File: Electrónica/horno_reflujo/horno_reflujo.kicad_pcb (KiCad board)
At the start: 2 copper layers, 39 parts, among them J2 5V USB cargador, J3 Nextion_touch_screen, J4 Max6675_modulo, J5 ESP01, J6 Alimentación y zc, J7 Relevador a ventilador, J8 Tarjeta a SSR, J9 SSR a resistencias, K1 SANYOU_SRD_Form_C, Q1 2N2222A-TO92, U1 SSR-40 DA, U2 LM7805CT, U3 74LS14, U4 LM7833CT, U5 ESP-01S

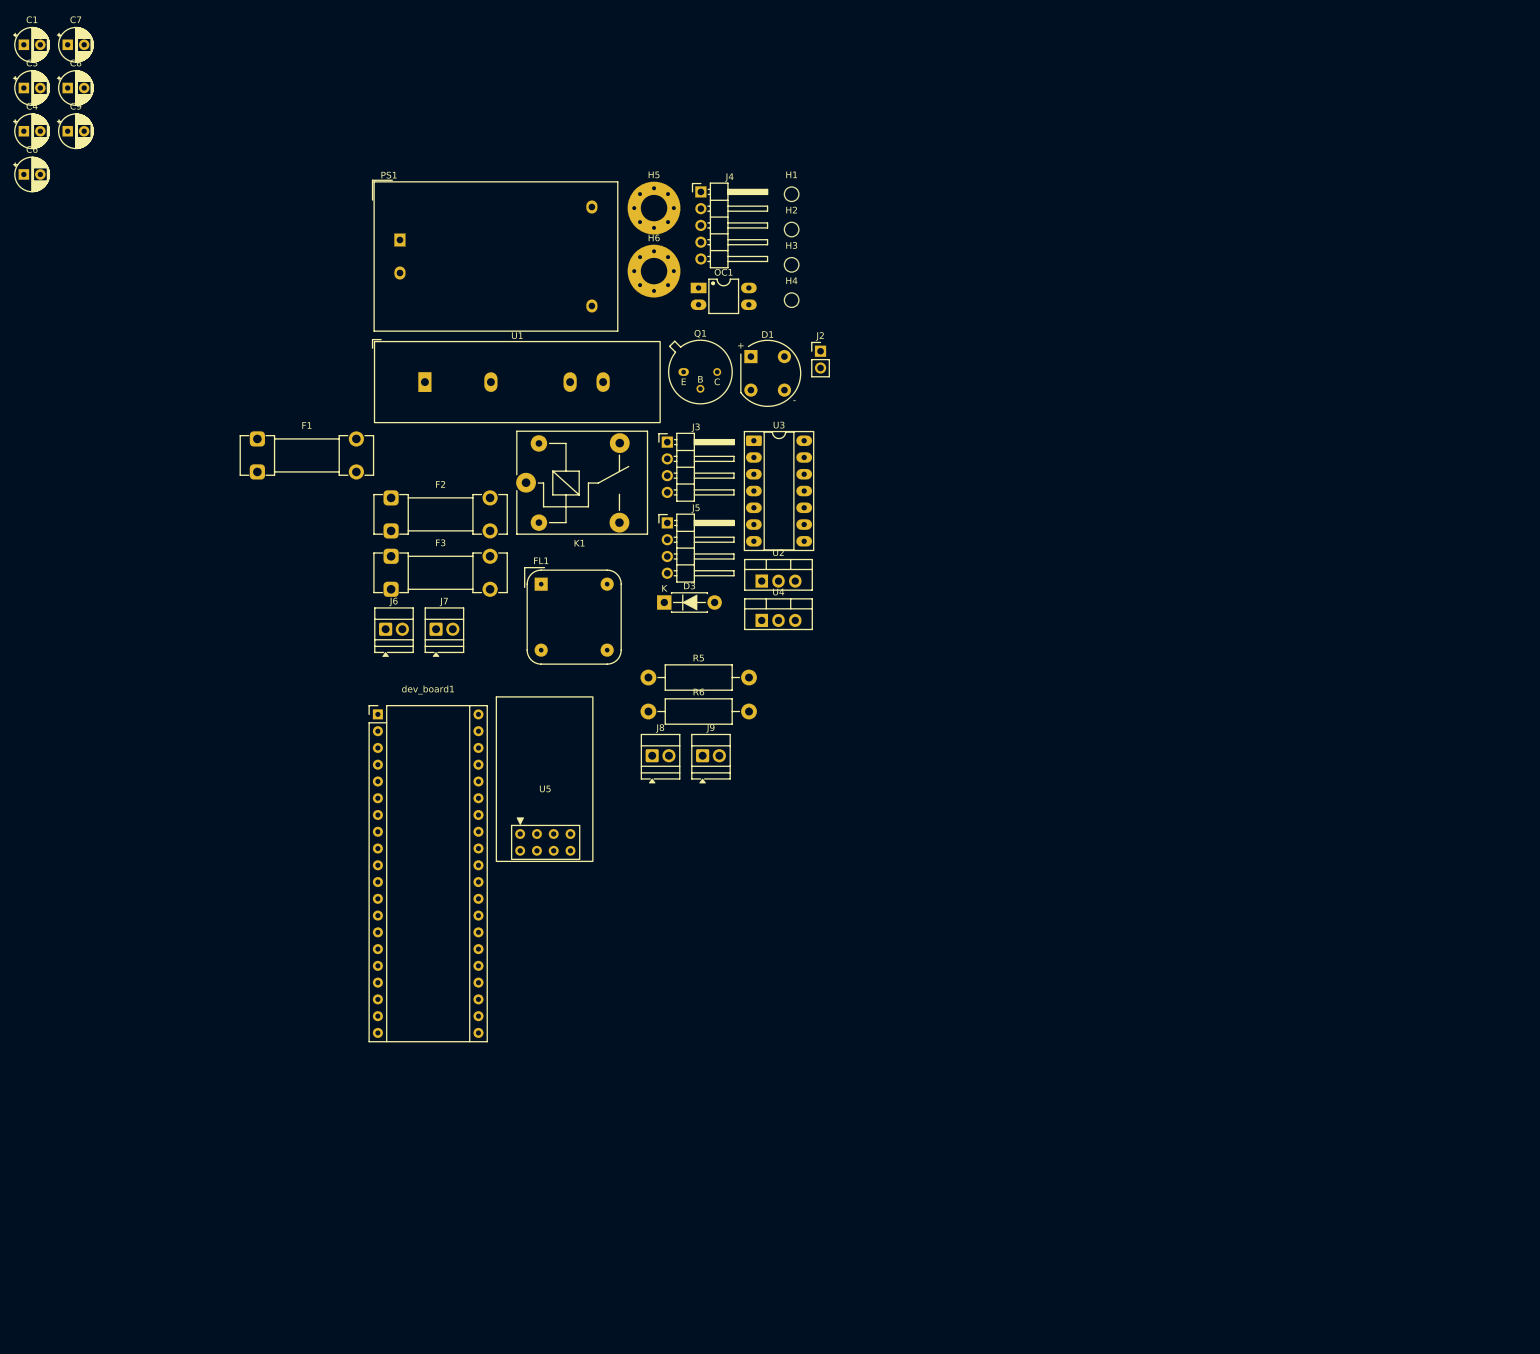
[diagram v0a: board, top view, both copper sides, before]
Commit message: pcb updated :)
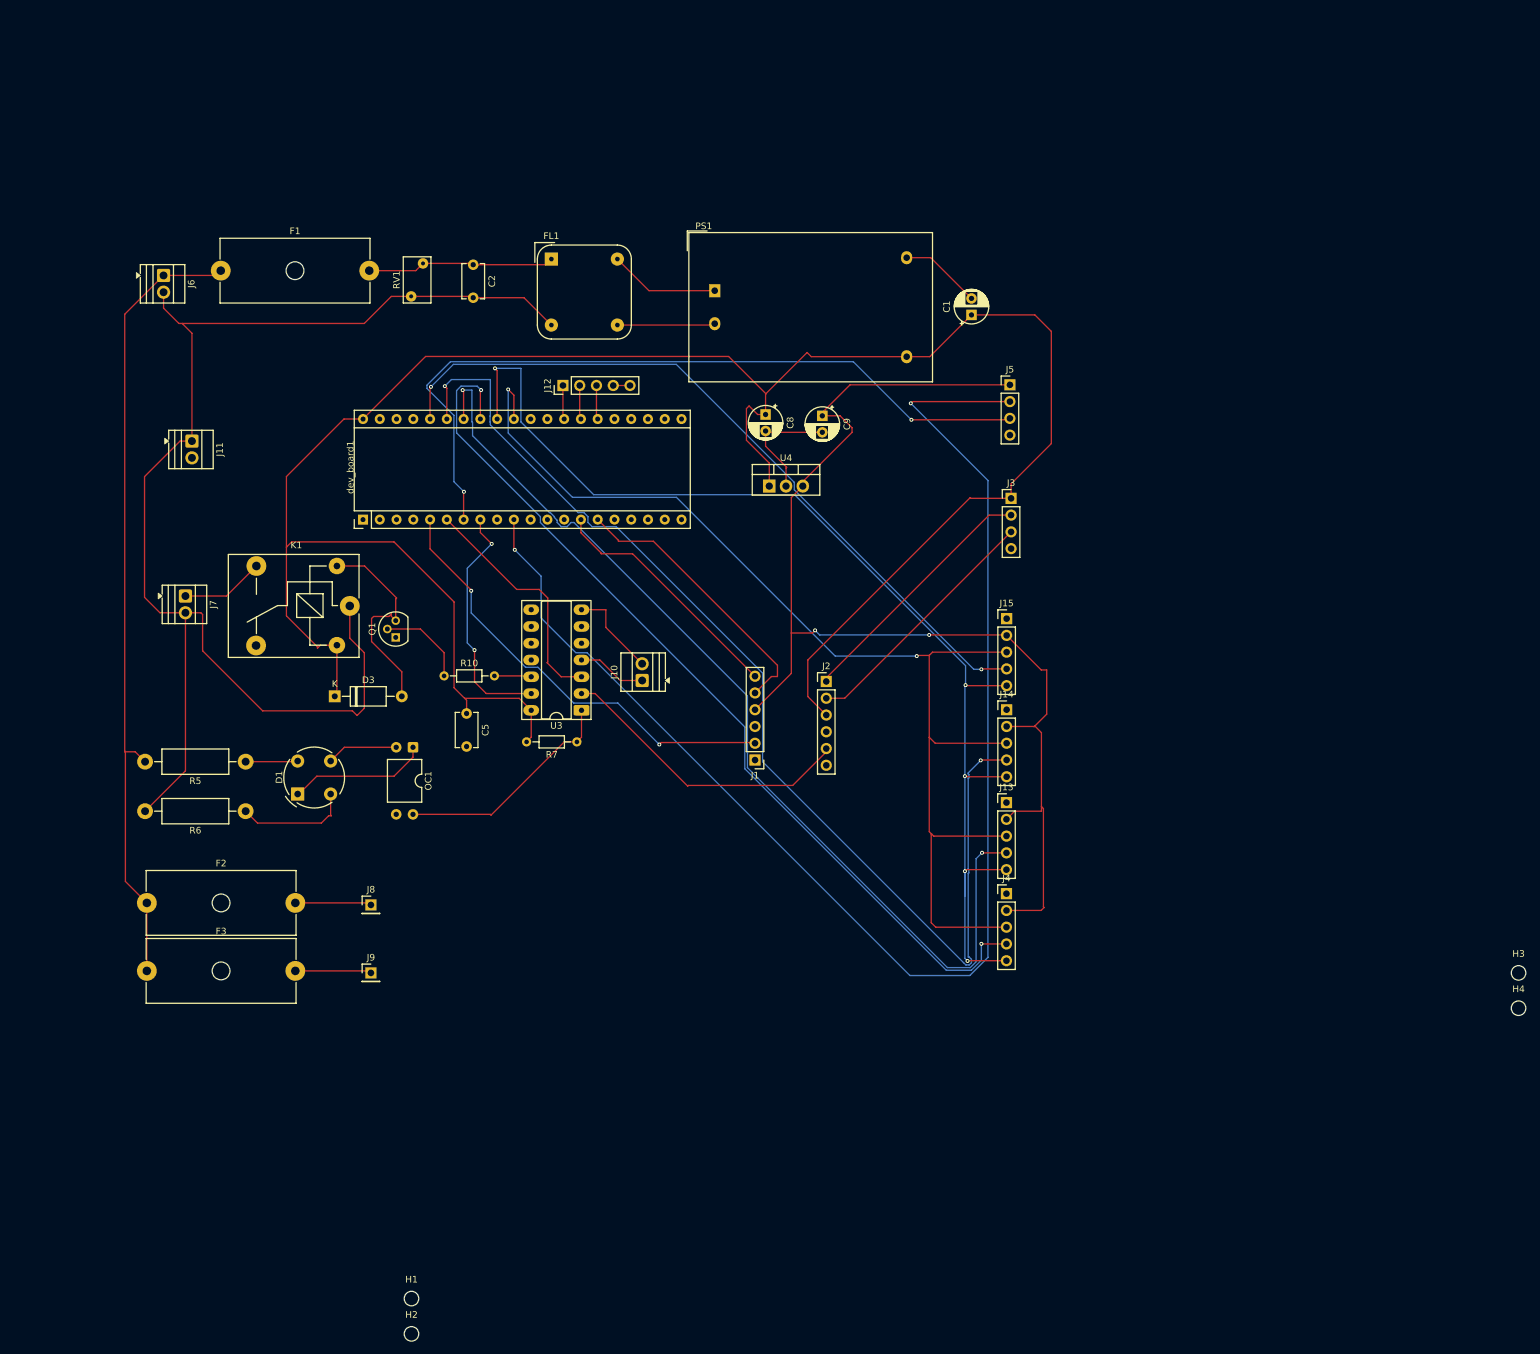
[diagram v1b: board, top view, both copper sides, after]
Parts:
- removed C3, C7: 1uf, Capacitor_THT:CP_Radial_D5.0mm_P2.50mm
- removed C4, C6: 10uf, Capacitor_THT:CP_Radial_D5.0mm_P2.50mm
- removed H5, H6: MountingHole_Pad_MP, MountingHole:MountingHole_4mm_Pad_Via
- removed U1: SSR-40 DA, Relay_THT:Relay_NCR_HHG1D-1
- removed U2: LM7805CT, PCM_Package_TO_SOT_THT_AKL:TO-220-3_Vertical
- removed U5: ESP-01S, RF_Module:ESP-01
- added C2: 0.1uF/275Vac, Capacitor_THT:C_Disc_D5.1mm_W3.2mm_P5.00mm, F.Cu at (69.7, 36.1)
- added C5: 100nf, Capacitor_THT:C_Disc_D5.1mm_W3.2mm_P5.00mm, F.Cu at (68.7, 104.1)
- added J1: LevelShifter, Connector_PinHeader_2.54mm:PinHeader_1x06_P2.54mm_Vertical, F.Cu at (112.4, 111.2)
- added J10: ssr1, TerminalBlock:TerminalBlock_Xinya_XY308-2.54-2P_1x02_P2.54mm_Horizontal, F.Cu at (95.3, 99.1)
- added J11: ssr2, TerminalBlock:TerminalBlock_Xinya_XY308-2.54-2P_1x02_P2.54mm_Horizontal, F.Cu at (27.1, 62.8)
- added J12: encoder, Connector_PinHeader_2.54mm:PinHeader_1x05_P2.54mm_Vertical, F.Cu at (83.3, 54.4)
- added J13: Max6675_modulo2, Connector_PinHeader_2.54mm:PinHeader_1x05_P2.54mm_Vertical, F.Cu at (150.5, 117.6)
- added J14: Max6675_modulo3, Connector_PinHeader_2.54mm:PinHeader_1x05_P2.54mm_Vertical, F.Cu at (150.5, 103.5)
- added J15: Max6675_modulo4, Connector_PinHeader_2.54mm:PinHeader_1x05_P2.54mm_Vertical, F.Cu at (150.5, 89.7)
- added R10: 1K, Resistor_THT:R_Axial_DIN0204_L3.6mm_D1.6mm_P7.62mm_Horizontal, F.Cu at (65.3, 98.4)
- added R7: 10K, Resistor_THT:R_Axial_DIN0204_L3.6mm_D1.6mm_P7.62mm_Horizontal, F.Cu at (85.4, 108.4)
- added RV1: 10D561K, Varistor:RV_Disc_D7mm_W4.2mm_P5mm, F.Cu at (62.1, 35.9)
- D1: footprint PCM_Diode_THT_AKL:Diode_Bridge_Round_D9.8mm -> Diode_THT:Diode_Bridge_Round_D9.0mm
- D3: footprint PCM_Diode_THT_AKL:D_DO-41_SOD81_P7.62mm_Horizontal -> Diode_THT:D_A-405_P10.16mm_Horizontal
- F1, F2, F3: footprint Fuse:Fuseholder_Clip-5x20mm_Schurter_OG_Lateral_P15.00x5.00mm_D1.3mm_Horizontal -> Fuse:Fuseholder_Cylinder-5x20mm_Schurter_0031_8201_Horizontal_Open
- J2: value 5V USB cargador -> LevelShifter; footprint Connector_PinHeader_2.54mm:PinHeader_1x02_P2.54mm_Vertical -> Connector_PinHeader_2.54mm:PinHeader_1x06_P2.54mm_Vertical
- J3: value Nextion_touch_screen -> Display Oled I2C; footprint Connector_PinHeader_2.54mm:PinHeader_1x04_P2.54mm_Horizontal -> Connector_PinHeader_2.54mm:PinHeader_1x04_P2.54mm_Vertical
- J4: footprint Connector_PinHeader_2.54mm:PinHeader_1x05_P2.54mm_Horizontal -> Connector_PinHeader_2.54mm:PinHeader_1x05_P2.54mm_Vertical
- J5: footprint Connector_PinHeader_2.54mm:PinHeader_1x04_P2.54mm_Horizontal -> Connector_PinHeader_2.54mm:PinHeader_1x04_P2.54mm_Vertical
- J8: value Tarjeta a SSR -> resistencia; footprint TerminalBlock:TerminalBlock_Xinya_XY308-2.54-2P_1x02_P2.54mm_Horizontal -> Connector_PinHeader_2.54mm:PinHeader_1x01_P2.54mm_Vertical
- J9: value SSR a resistencias -> resistencia1; footprint TerminalBlock:TerminalBlock_Xinya_XY308-2.54-2P_1x02_P2.54mm_Horizontal -> Connector_PinHeader_2.54mm:PinHeader_1x01_P2.54mm_Vertical
- OC1: footprint PCM_Package_DIP_AKL:DIP-4_W7.62mm_LongPads -> Package_DIP:DIP-4_W10.16mm
- Q1: footprint PCM_Package_TO_SOT_THT_AKL:TO-39-3_EBC -> Package_TO_SOT_THT:TO-92
- U4: footprint PCM_Package_TO_SOT_THT_AKL:TO-220-3_Vertical -> Package_TO_SOT_THT:TO-220-3_Vertical
- moved H1 177.0 mm to (60.4, 192.8)
- moved H2 177.0 mm to (60.4, 198.1)
- moved H3 153.8 mm to (228.1, 143.4)
- moved H4 153.8 mm to (228.1, 148.8)
- moved C1 149.3 mm to (145.2, 43.7), turned to 90 degrees
- moved C9 122.2 mm to (122.6, 59.0), turned to -90 degrees
- moved C8 116.7 mm to (114.0, 58.8), turned to -90 degrees
- moved J4 116.0 mm to (150.5, 131.4)
- moved D1 95.4 mm to (43.1, 116.3), turned to 90 degrees
- moved OC1 82.0 mm to (60.6, 109.2), turned to -90 degrees
- moved F3 72.9 mm to (20.2, 143.1)
- moved F2 71.7 mm to (20.2, 132.8)
- moved J6 63.3 mm to (22.8, 37.7), turned to -90 degrees
- moved R6 62.9 mm to (35.2, 118.9), turned to 180 degrees
- moved R5 62.3 mm to (35.2, 111.4), turned to 180 degrees
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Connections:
- F2 pad 2: Net-(F2-Pad2) -> Net-(J8-Pin_1)
- F3 pad 2: Net-(F3-Pad2) -> Net-(J9-Pin_1)
- J2 pad 1: GND -> Net-(J2-Pin_1)
- J2 pad 2: +5V -> Net-(J2-Pin_2)
- J3 pad 2: Net-(J3-Pin_2) -> Net-(J2-Pin_1)
- J3 pad 3: Net-(J3-Pin_3) -> Net-(J2-Pin_2)
- J4 pad 2: +5V -> +3.3V
- J4 pad 3: /sck -> SPI1_SCK
- J4 pad 4: /cs -> CS_0
- J4 pad 5: /so -> SPI1_MISO
- J8 pad 1: /SSR_led -> Net-(J8-Pin_1)
- J9 pad 1: unconnected-(J9-Pin_1-Pad1) -> Net-(J9-Pin_1)
- U3 pad 10: unconnected-(U3-Pad10) -> (no net)
- U3 pad 11: GND -> (no net)
- U3 pad 2: Net-(R8-Pad2) -> zero
- U3 pad 4: /SSR_led -> Net-(J10-Pin_1)
- U3 pad 5: /Tx_mcu_screen -> (no net)
- U3 pad 6: Net-(U3-Pad6) -> (no net)
- U3 pad 8: Net-(J3-Pin_3) -> (no net)
- U3 pad 9: Net-(U3-Pad6) -> (no net)
- dev_board1 pad 10: unconnected-(dev_board1-A15-Pad10) -> /Rx_mcu_esp01
- dev_board1 pad 14: unconnected-(dev_board1-B6-Pad14) -> I2C1_SCL
- dev_board1 pad 15: unconnected-(dev_board1-B7-Pad15) -> I2C1_SDA
- dev_board1 pad 22: unconnected-(dev_board1-C13-Pad22) -> built_in_led
- dev_board1 pad 26: unconnected-(dev_board1-A0-Pad26) -> ENCODER_A
- dev_board1 pad 27: unconnected-(dev_board1-A1-Pad27) -> ENCODER_B
- dev_board1 pad 28: unconnected-(dev_board1-A2-Pad28) -> ENCODER_BTN
- dev_board1 pad 31: unconnected-(dev_board1-A5-Pad31) -> SPI1_SCK
- dev_board1 pad 32: unconnected-(dev_board1-A6-Pad32) -> SPI1_MISO
- dev_board1 pad 33: unconnected-(dev_board1-A7-Pad33) -> CS_0
- dev_board1 pad 34: unconnected-(dev_board1-B0-Pad34) -> CS_1
- dev_board1 pad 35: unconnected-(dev_board1-B1-Pad35) -> CS_2
- dev_board1 pad 36: unconnected-(dev_board1-B2-Pad36) -> CS_3
- dev_board1 pad 5: unconnected-(dev_board1-A8-Pad5) -> /zc
- dev_board1 pad 6: unconnected-(dev_board1-A9-Pad6) -> /fire
- dev_board1 pad 7: unconnected-(dev_board1-A10-Pad7) -> /Tx_mcu_esp01
- dev_board1 pad 8: unconnected-(dev_board1-A11-Pad8) -> /fan
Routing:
- net +5V: track 0.00 -> 332.7 mm
- net /Rx_mcu_esp01: track 0.00 -> 211.8 mm, vias 0 -> 2
- net NEUT: track 0.00 -> 205.2 mm
- net +3.3V: track 0.00 -> 180.1 mm, vias 0 -> 2
- net SPI1_SCK: track 0.00 -> 177.1 mm, vias 0 -> 2
- net SPI1_MISO: track 0.00 -> 176.2 mm, vias 0 -> 5
- net CS_2: track 0.00 -> 170.5 mm, vias 0 -> 2
- net CS_1: track 0.00 -> 150.6 mm, vias 0 -> 2
- net CS_0: track 0.00 -> 139.5 mm, vias 0 -> 2
- net LINE: track 0.00 -> 122.0 mm
- net /Tx_mcu_esp01: track 0.00 -> 116.2 mm, vias 0 -> 2
- net CS_3: track 0.00 -> 113.4 mm, vias 0 -> 2
- net /zc: track 0.00 -> 68.6 mm, vias 0 -> 2
- net GND: track 0.00 -> 47.5 mm
- net zero: track 0.00 -> 45.3 mm
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
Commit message: actualización del main
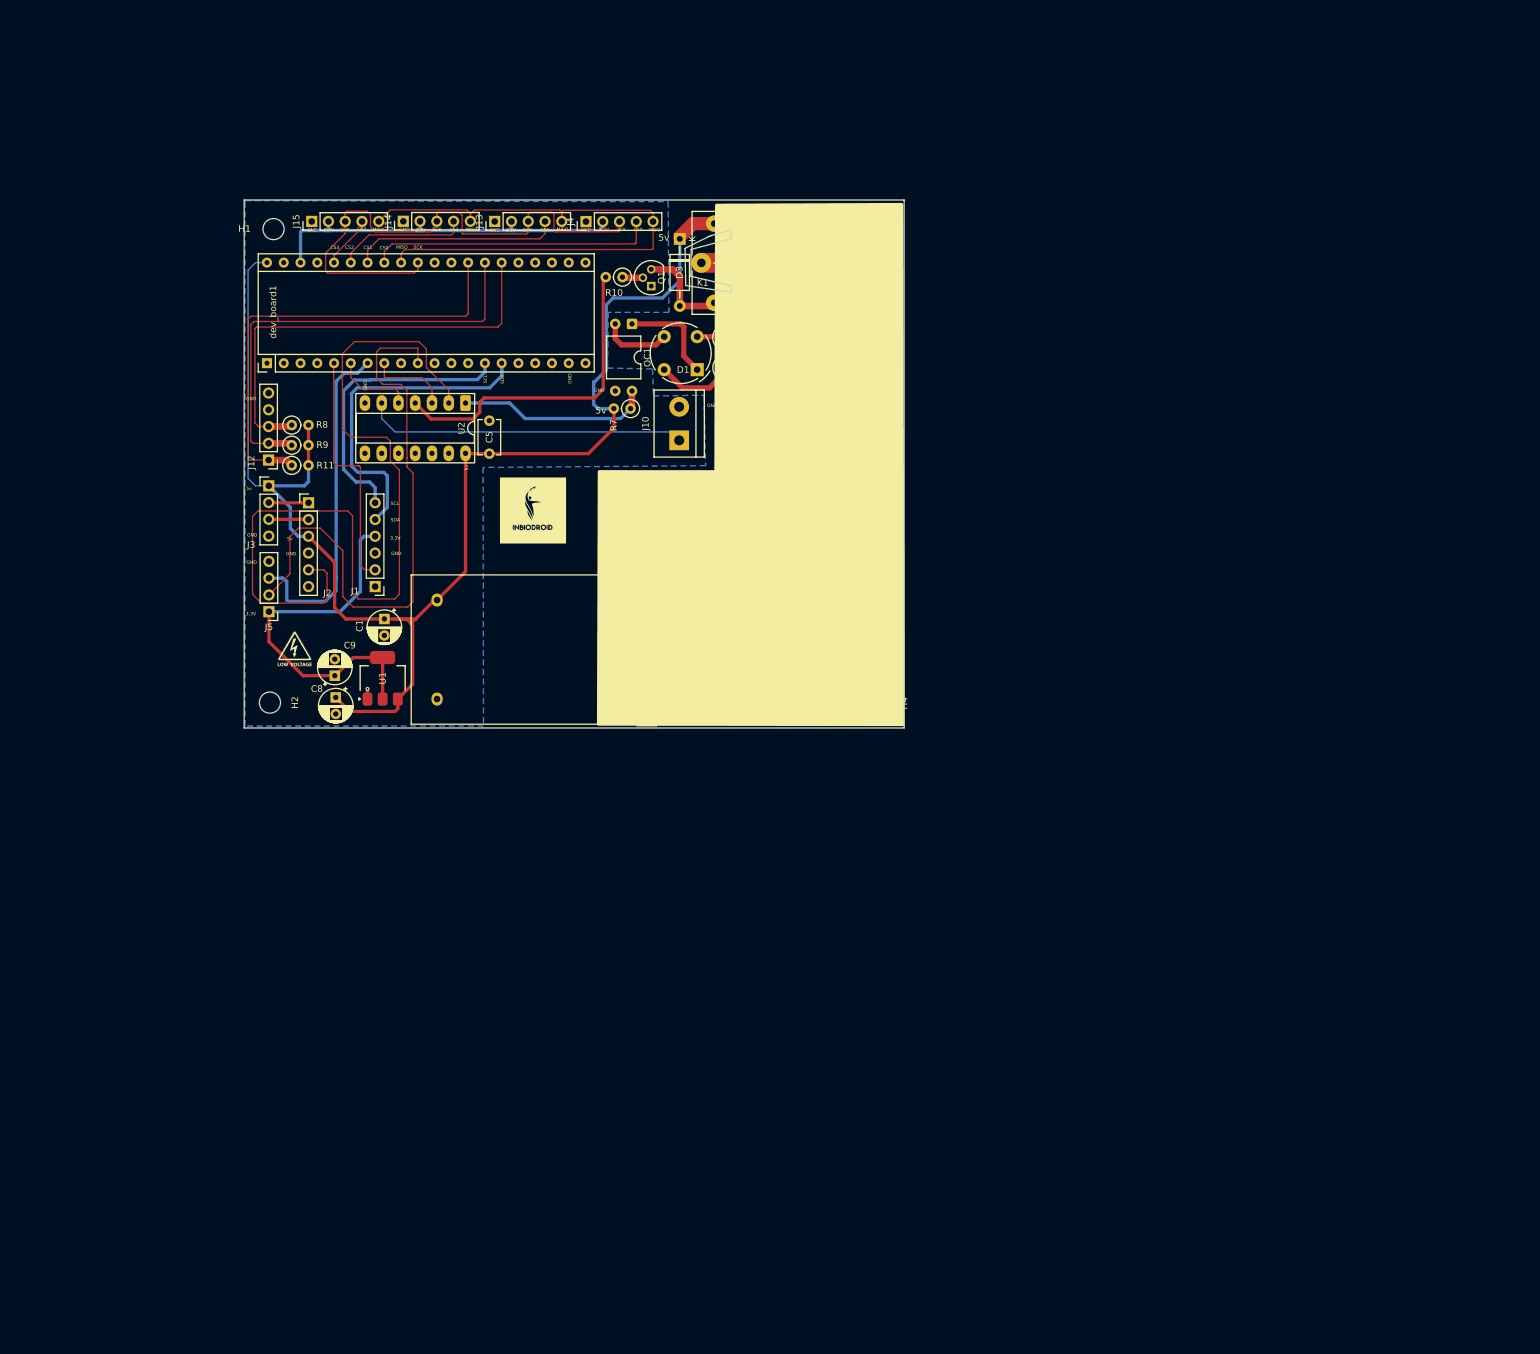
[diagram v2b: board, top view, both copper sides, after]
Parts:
- removed F3: 15A, Fuse:Fuseholder_Cylinder-5x20mm_Schurter_0031_8201_Horizontal_Open
- removed J9: resistencia1, Connector_PinHeader_2.54mm:PinHeader_1x01_P2.54mm_Vertical
- removed U3: 74LS14, Package_DIP:DIP-14_W7.62mm_Socket_LongPads
- removed U4: LM7833CT, Package_TO_SOT_THT:TO-220-3_Vertical
- added G***: LOGO, LOGO, F.Cu at (97.5, 74.9)
- added G***: LOGO, LOGO, F.Cu at (78.8, 73.3)
- added G***: LOGO, LOGO, F.Cu at (42.5, 94.2)
- added R11: 10K, Resistor_THT:R_Axial_DIN0207_L6.3mm_D2.5mm_P2.54mm_Vertical, F.Cu at (42.2, 66.5)
- added R8: 10K, Resistor_THT:R_Axial_DIN0207_L6.3mm_D2.5mm_P2.54mm_Vertical, F.Cu at (42.2, 60.4)
- added R9: 10K, Resistor_THT:R_Axial_DIN0207_L6.3mm_D2.5mm_P2.54mm_Vertical, F.Cu at (42.2, 63.5)
- added U1: LD1117S33TR_SOT223, Package_TO_SOT_SMD:SOT-223-3_TabPin2, F.Cu at (56.0, 98.8)
- added U2: 74LS14, Package_DIP:DIP-14_W7.62mm_Socket_LongPads, F.Cu at (68.5, 57.1)
- H1, H2, H3, H4: footprint MountingHole:MountingHole_2.2mm_M2_DIN965 -> MountingHole:MountingHole_3.2mm_M3_DIN965
- J10, J11, J6, J7: footprint TerminalBlock:TerminalBlock_Xinya_XY308-2.54-2P_1x02_P2.54mm_Horizontal -> TerminalBlock:TerminalBlock_bornier-2_P5.08mm
- R10, R7: footprint Resistor_THT:R_Axial_DIN0204_L3.6mm_D1.6mm_P7.62mm_Horizontal -> Resistor_THT:R_Axial_DIN0207_L6.3mm_D2.5mm_P2.54mm_Vertical
- R5, R6: footprint Resistor_THT:R_Axial_DIN0411_L9.9mm_D3.6mm_P15.24mm_Horizontal -> Resistor_THT:R_Axial_DIN0411_L9.9mm_D3.6mm_P5.08mm_Vertical
- moved H1 163.4 mm to (39.5, 30.7), turned to 180 degrees
- moved H3 148.6 mm to (131.8, 30.3), turned to 180 degrees
- moved F2 128.8 mm to (133.3, 71.2), turned to 180 degrees
- moved J6 122.6 mm to (130.9, 95.6), turned to 90 degrees
- moved J15 121.3 mm to (45.2, 29.5), turned to 90 degrees
- moved J4 120.1 mm to (86.8, 29.6), turned to 90 degrees
- moved J14 117.6 mm to (59.1, 29.5), turned to 90 degrees
- moved J5 117.4 mm to (38.8, 88.7), turned to 180 degrees
- moved J13 117.3 mm to (73.0, 29.5), turned to 90 degrees
- moved J7 112.5 mm to (127.0, 36.4)
- moved J3 112.5 mm to (38.7, 69.6)
- moved F1 111.2 mm to (133.3, 81.6), turned to 180 degrees
- moved H4 107.3 mm to (131.2, 102.5), turned to -90 degrees
- moved R6 102.1 mm to (107.9, 47.2), turned to 0 degrees
- moved C1 100.2 mm to (56.2, 89.8), turned to -90 degrees
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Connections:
- J13 pad 2: +3.3V -> +3.3Vmc
- J14 pad 2: +3.3V -> +3.3Vmc
- J15 pad 2: +3.3V -> +3.3Vmc
- J4 pad 2: +3.3V -> +3.3Vmc
- J6 pad 1: LINE -> NEUT
- J6 pad 2: NEUT -> LINE
- J7 pad 2: NEUT -> LINE
- R5 pad 2: LINE -> Net-(J8-Pin_1)
- dev_board1 pad 38: unconnected-(dev_board1-3.3-Pad38) -> +3.3Vmc
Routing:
- net CS_2: track 170.5 -> 20.0 mm, vias 2 -> 0
- net /Rx_mcu_esp01: track 211.8 -> 89.3 mm, vias 2 -> 0
- net +3.3V: track 180.1 -> 57.8 mm, vias 2 -> 0
- net CS_1: track 150.6 -> 31.7 mm, vias 2 -> 0
- net +5V: track 332.7 -> 219.8 mm
- net CS_3: track 113.4 -> 7.99 mm, vias 2 -> 0
- net CS_0: track 139.5 -> 43.6 mm, vias 2 -> 0
- net SPI1_SCK: track 177.1 -> 83.7 mm, vias 2 -> 0
- net zero: track 45.3 -> 133.0 mm
- net SPI1_MISO: track 176.2 -> 93.6 mm, vias 5 -> 0
- net ENCODER_BTN: track 5.16 -> 69.6 mm
- net /Tx_mcu_esp01: track 116.2 -> 51.9 mm, vias 2 -> 0
- net ENCODER_B: track 5.16 -> 68.5 mm
- net ENCODER_A: track 5.16 -> 67.1 mm
- net +3.3Vmc: track 0.00 -> 58.1 mm
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- added copper zone on B.Cu, net GND
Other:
- board outline added: 100 x 80 mm
- board text added: "3.3V"
- board text added: "5v"
- board text added: "CS0"
- board text added: "CS1"
- board text added: "CS2"
- board text added: "CS3"
- board text added: "GND"
- board text added: "LINE VENT"
- board text added: "MISO"
- board text added: "NEUT LINE"
- board text added: "NEUT SSR"
- board text added: "RESISTENCIA"
- board text added: "SCK"
- board text added: "SCL"
- board text added: "SDA"
